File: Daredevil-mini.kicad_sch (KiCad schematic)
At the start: 55 parts, among them J1 USB_A, SW1 KMR221GLFS, Y1 ABM8-272-T3

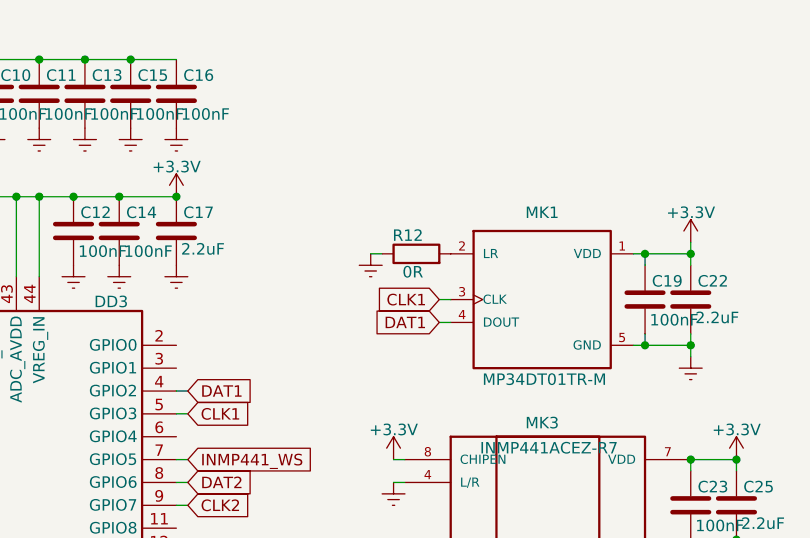
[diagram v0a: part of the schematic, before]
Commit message: udp PCB
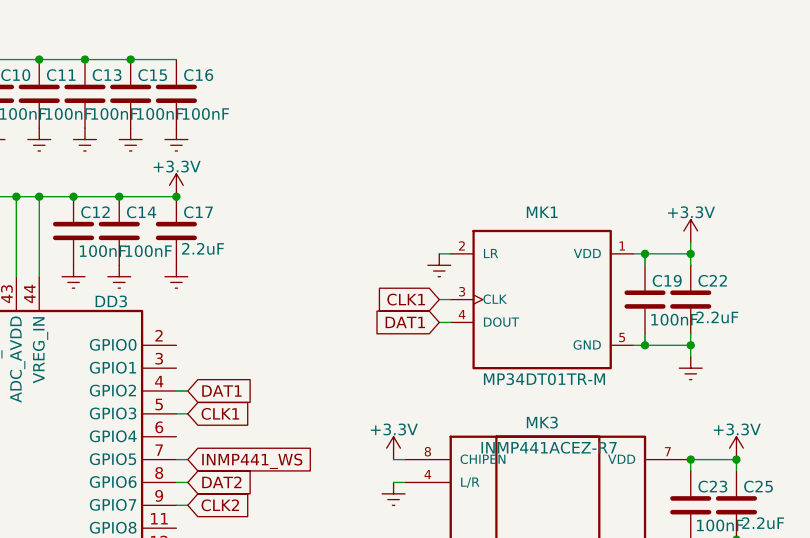
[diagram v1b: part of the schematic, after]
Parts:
- removed R12: 0R, PCM_Resistor_SMD_AKL:R_0201_0603Metric, symbol Device:R
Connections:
- net Earth: now also MK1.2 (LR)

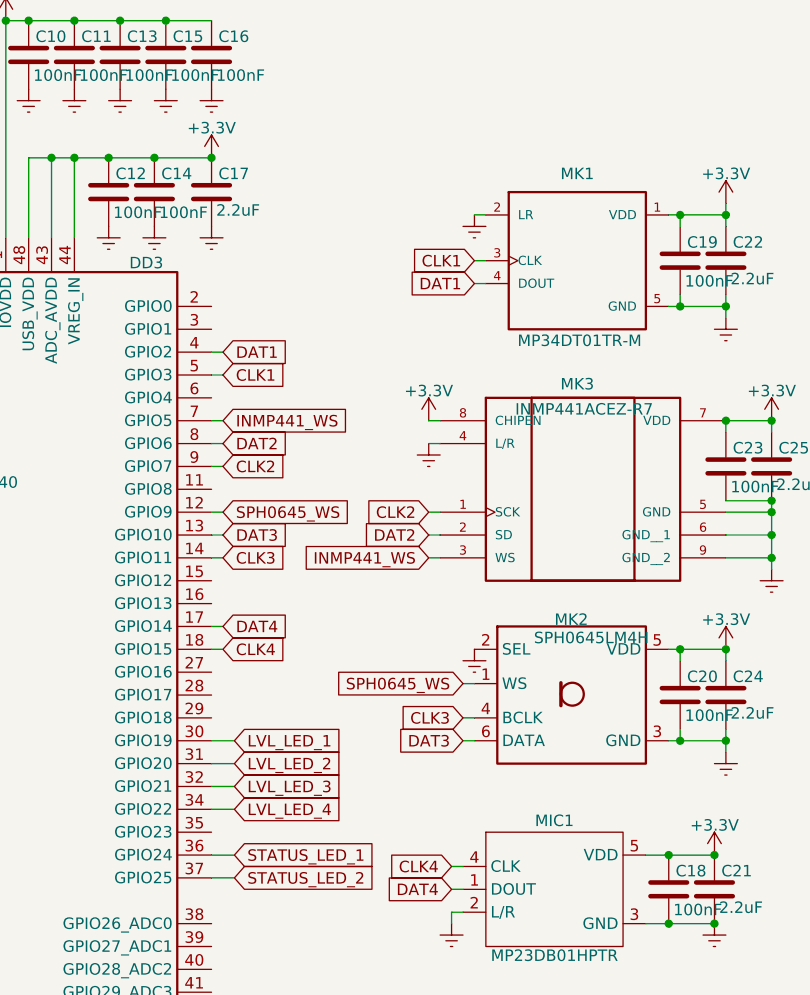
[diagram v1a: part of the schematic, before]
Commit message: rev0 ready
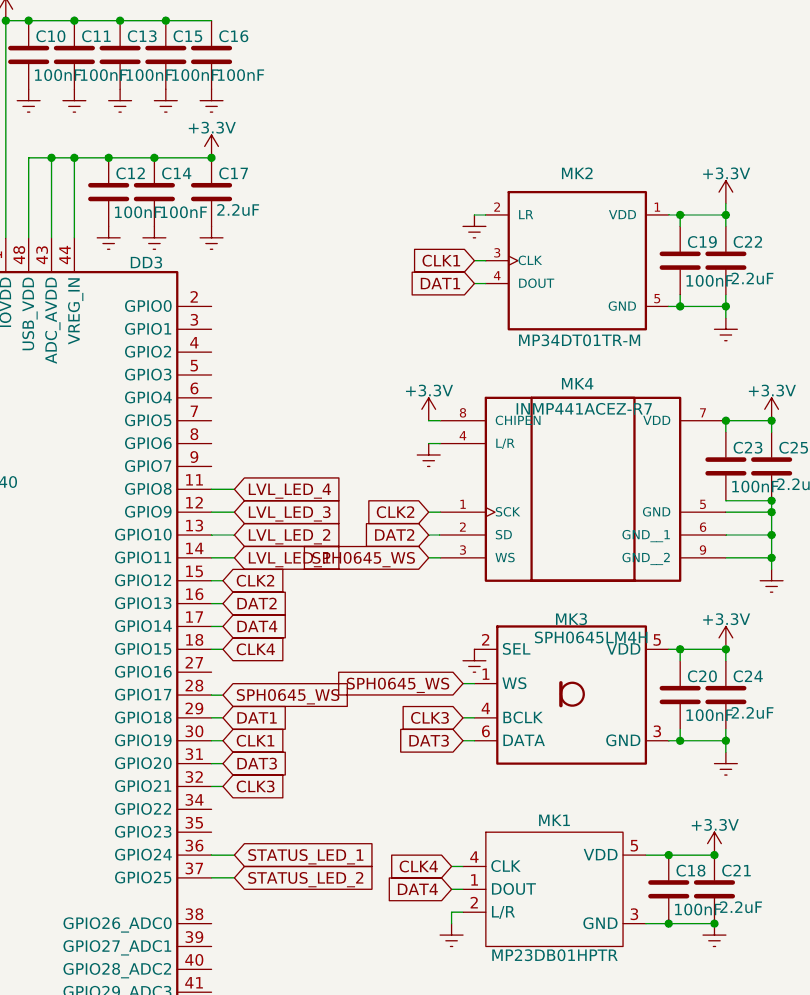
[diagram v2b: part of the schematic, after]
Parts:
- renumbered MIC1 to MK1, MK1 to MK2, MK2 to MK3, MK3 to MK4
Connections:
- net CLK1: now also DD3.30 (GPIO19); no longer DD3.5 (GPIO3)
- net CLK2: now also DD3.15 (GPIO12); no longer DD3.9 (GPIO7)
- net CLK3: now also DD3.32 (GPIO21); no longer DD3.14 (GPIO11)
- net DAT1: now also DD3.29 (GPIO18); no longer DD3.4 (GPIO2)
- net DAT2: now also DD3.16 (GPIO13); no longer DD3.8 (GPIO6)
- net DAT3: now also DD3.31 (GPIO20); no longer DD3.13 (GPIO10)
- net LVL_LED_1: now also DD3.14 (GPIO11); no longer DD3.30 (GPIO19)
- net LVL_LED_2: now also DD3.13 (GPIO10); no longer DD3.31 (GPIO20)
- net LVL_LED_3: now also DD3.12 (GPIO9); no longer DD3.32 (GPIO21)
- net LVL_LED_4: now also DD3.11 (GPIO8); no longer DD3.34 (GPIO22)
- net SPH0645_WS: now also DD3.28 (GPIO17), MK4.3 (WS); no longer DD3.12 (GPIO9)
- net INMP441_WS: no longer names the net of DD3.7 (GPIO5)
- net INMP441_WS: no longer MK4.3 (WS)
